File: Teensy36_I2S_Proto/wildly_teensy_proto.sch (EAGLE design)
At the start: 25 parts, among them CON1 MIKROE_BUS_CONN, SW2 Push_Button

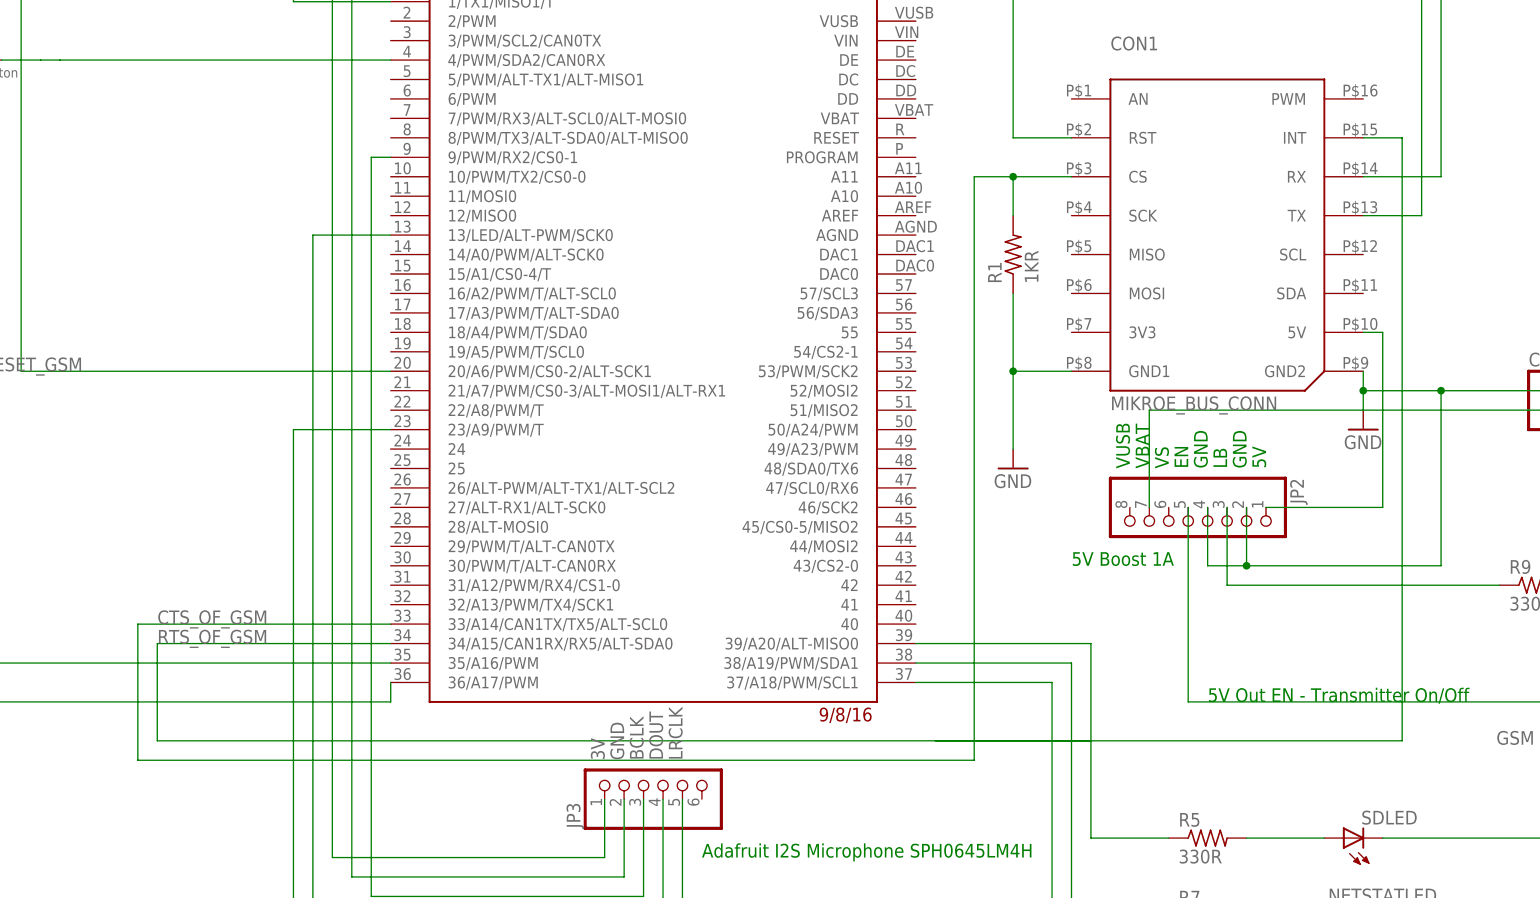
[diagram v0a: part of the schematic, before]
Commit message: Fix/Swap RTS and CTS connections
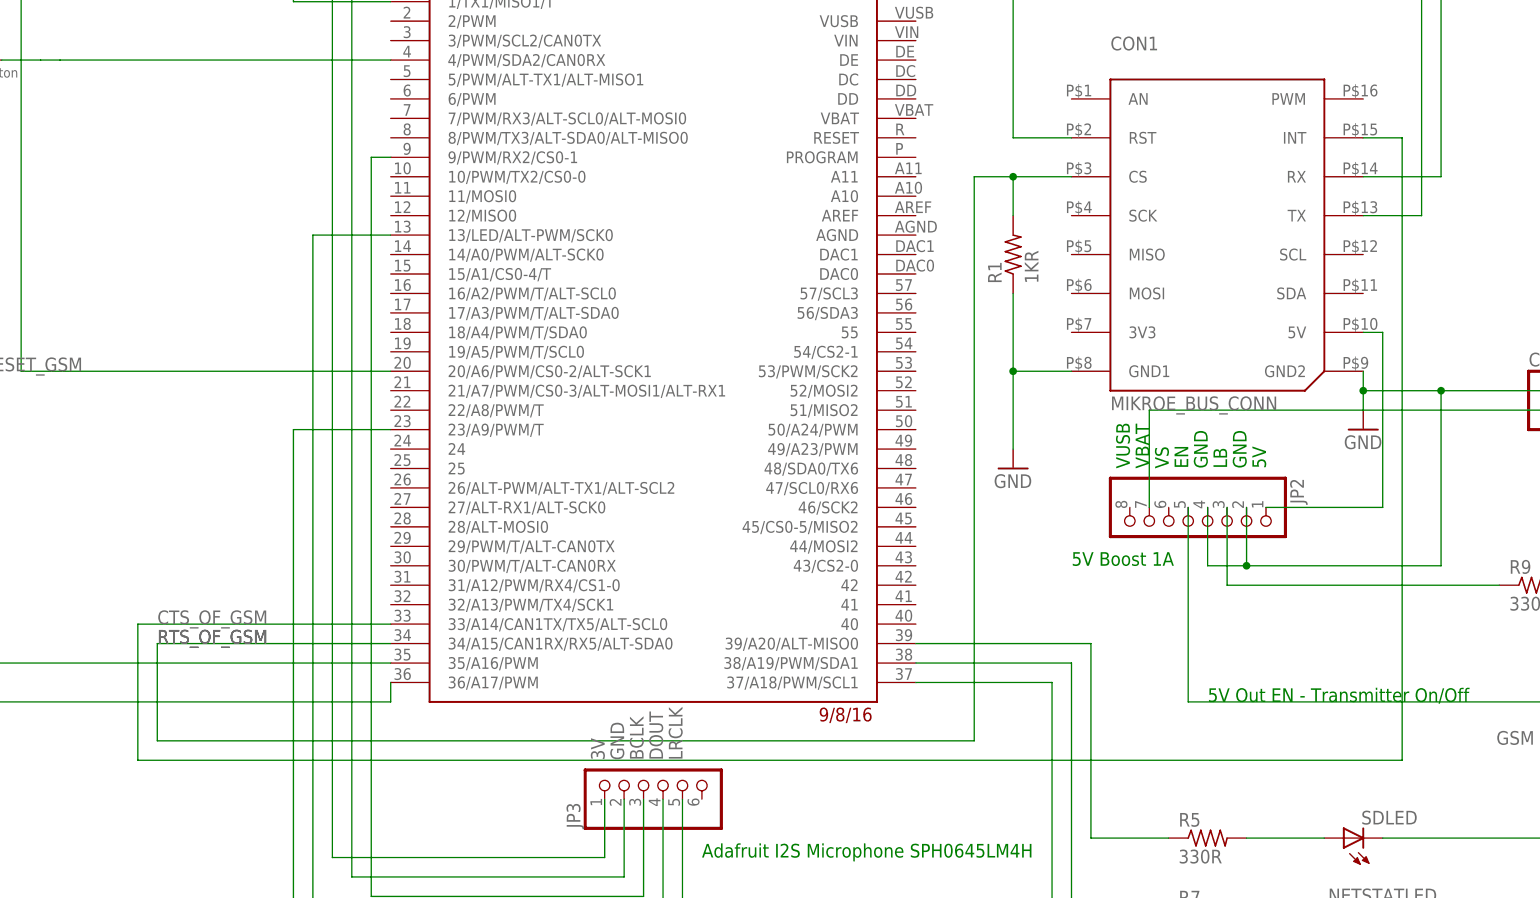
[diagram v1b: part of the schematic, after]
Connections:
- net CTS_OF_GSM: now also CON1.INT; no longer CON1.CS, R1.2
- net RTS_OF_GSM: now also CON1.CS, R1.2; no longer CON1.INT
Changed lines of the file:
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@@
 <net name="CTS_OF_GSM" class="0">
 <segment>
+<wire x1="162.56" y1="-15.24" x2="162.56" y2="66.04" width="0.1524" layer="91"/>
+<pinref part="CON1" gate="G$1" pin="INT"/>
+<wire x1="162.56" y1="66.04" x2="157.48" y2="66.04" width="0.1524" layer="91"/>
 <pinref part="U$1" gate="G$1" pin="33/A14/CAN1TX/TX5/ALT-SCL0"/>
 <wire x1="30.48" y1="2.54" x2="-2.54" y2="2.54" width="0.1524" layer="91"/>
 <label x="0" y="2.54" size="1.778" layer="95"/>
 <wire x1="-2.54" y1="2.54" x2="-2.54" y2="-15.24" width="0.1524" layer="91"/>
-<wire x1="-2.54" y1="-15.24" x2="106.68" y2="-15.24" width="0.1524" layer="91"/>
-<pinref part="CON1" gate="G$1" pin="CS"/>
-<wire x1="119.38" y1="60.96" x2="111.76" y2="60.96" width="0.1524" layer="91"/>
-<wire x1="111.76" y1="60.96" x2="106.68" y2="60.96" width="0.1524" layer="91"/>
-<wire x1="106.68" y1="60.96" x2="106.68" y2="-15.24" width="0.1524" layer="91"/>
-<pinref part="R1" gate="G$1" pin="2"/>
-<wire x1="111.76" y1="55.88" x2="111.76" y2="60.96" width="0.1524" layer="91"/>
-<junction x="111.76" y="60.96"/>
+<wire x1="-2.54" y1="-15.24" x2="162.56" y2="-15.24" width="0.1524" layer="91"/>
 </segment>
 </net>
 <net name="RTS_OF_GSM" class="0">
 <segment>
+<label x="0" y="0" size="1.778" layer="95"/>
+</segment>
+<segment>
 <pinref part="U$1" gate="G$1" pin="34/A15/CAN1RX/RX5/ALT-SDA0"/>
 <wire x1="30.48" y1="0" x2="0" y2="0" width="0.1524" layer="91"/>
+<wire x1="0" y1="0" x2="0" y2="-12.7" width="0.1524" layer="91"/>
+<wire x1="0" y1="-12.7" x2="106.68" y2="-12.7" width="0.1524" layer="91"/>
+<pinref part="CON1" gate="G$1" pin="CS"/>
+<wire x1="119.38" y1="60.96" x2="111.76" y2="60.96" width="0.1524" layer="91"/>
+<wire x1="111.76" y1="60.96" x2="106.68" y2="60.96" width="0.1524" layer="91"/>
+<junction x="111.76" y="60.96"/>
+<pinref part="R1" gate="G$1" pin="2"/>
+<wire x1="111.76" y1="55.88" x2="111.76" y2="60.96" width="0.1524" layer="91"/>
+<wire x1="106.68" y1="-12.7" x2="106.68" y2="60.96" width="0.1524" layer="91"/>
 <label x="0" y="0" size="1.778" layer="95"/>
-<wire x1="0" y1="0" x2="0" y2="-12.7" width="0.1524" layer="91"/>
-<wire x1="0" y1="-12.7" x2="162.56" y2="-12.7" width="0.1524" layer="91"/>
-<wire x1="162.56" y1="-12.7" x2="162.56" y2="66.04" width="0.1524" layer="91"/>
-<pinref part="CON1" gate="G$1" pin="INT"/>
-<wire x1="162.56" y1="66.04" x2="157.48" y2="66.04" width="0.1524" layer="91"/>
 </segment>
 </net>
@@
 </segment>
 </net>
-<net name="N$22" class="0">
-<segment>
-<wire x1="101.6" y1="-12.7" x2="121.92" y2="-12.7" width="0.1524" layer="91"/>
-</segment>
-</net>
